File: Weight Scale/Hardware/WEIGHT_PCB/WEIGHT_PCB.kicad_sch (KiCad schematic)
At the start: 0 parts

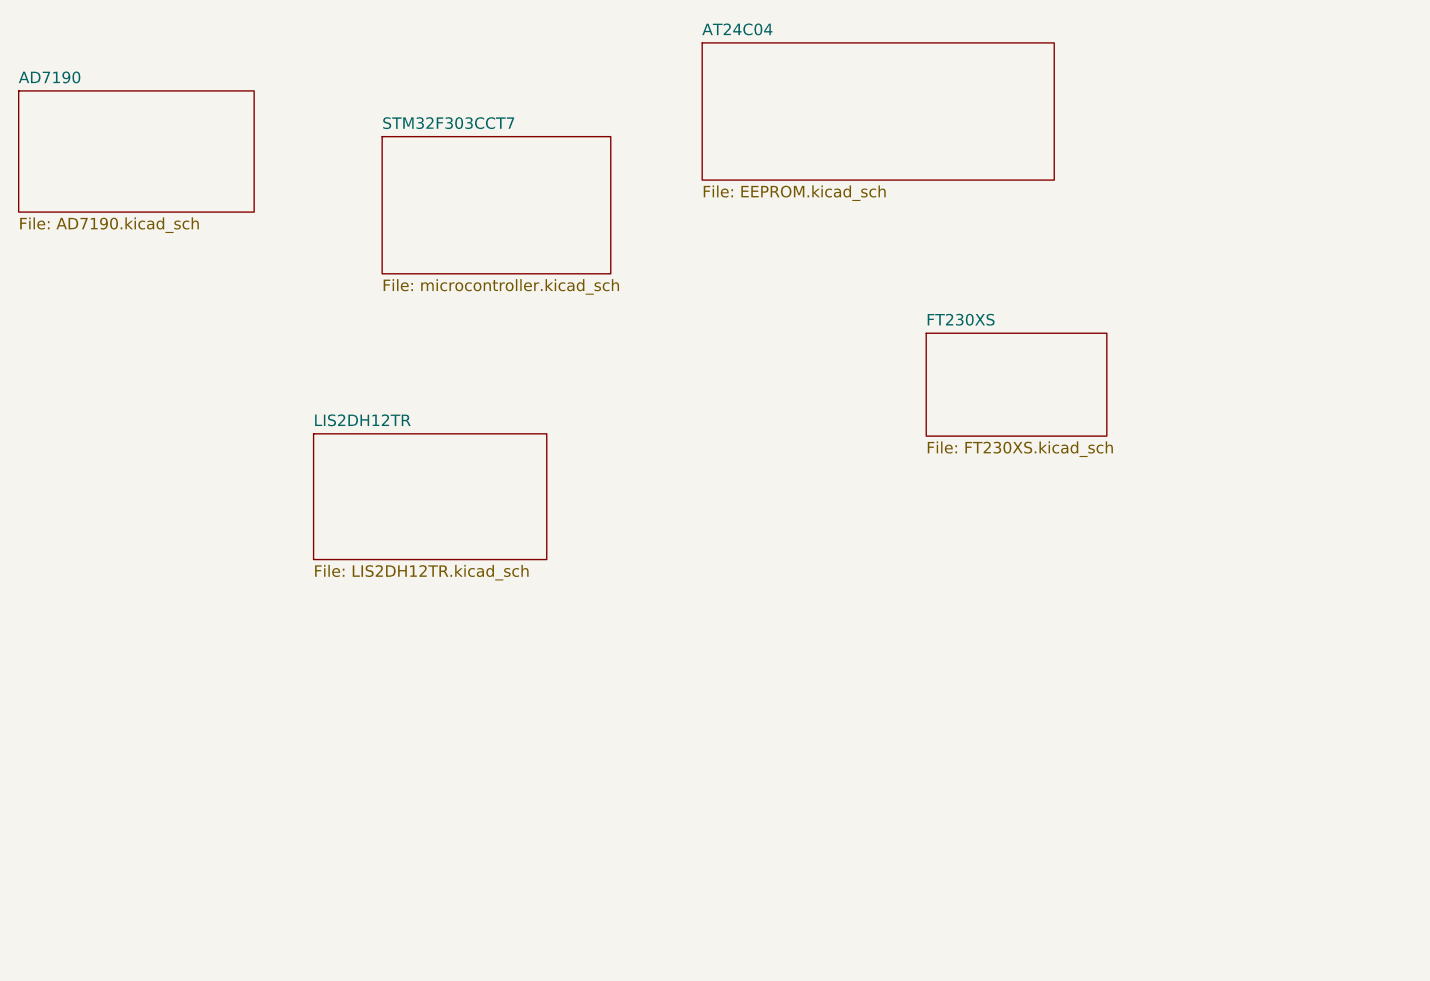
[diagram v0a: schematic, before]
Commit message: update schematics
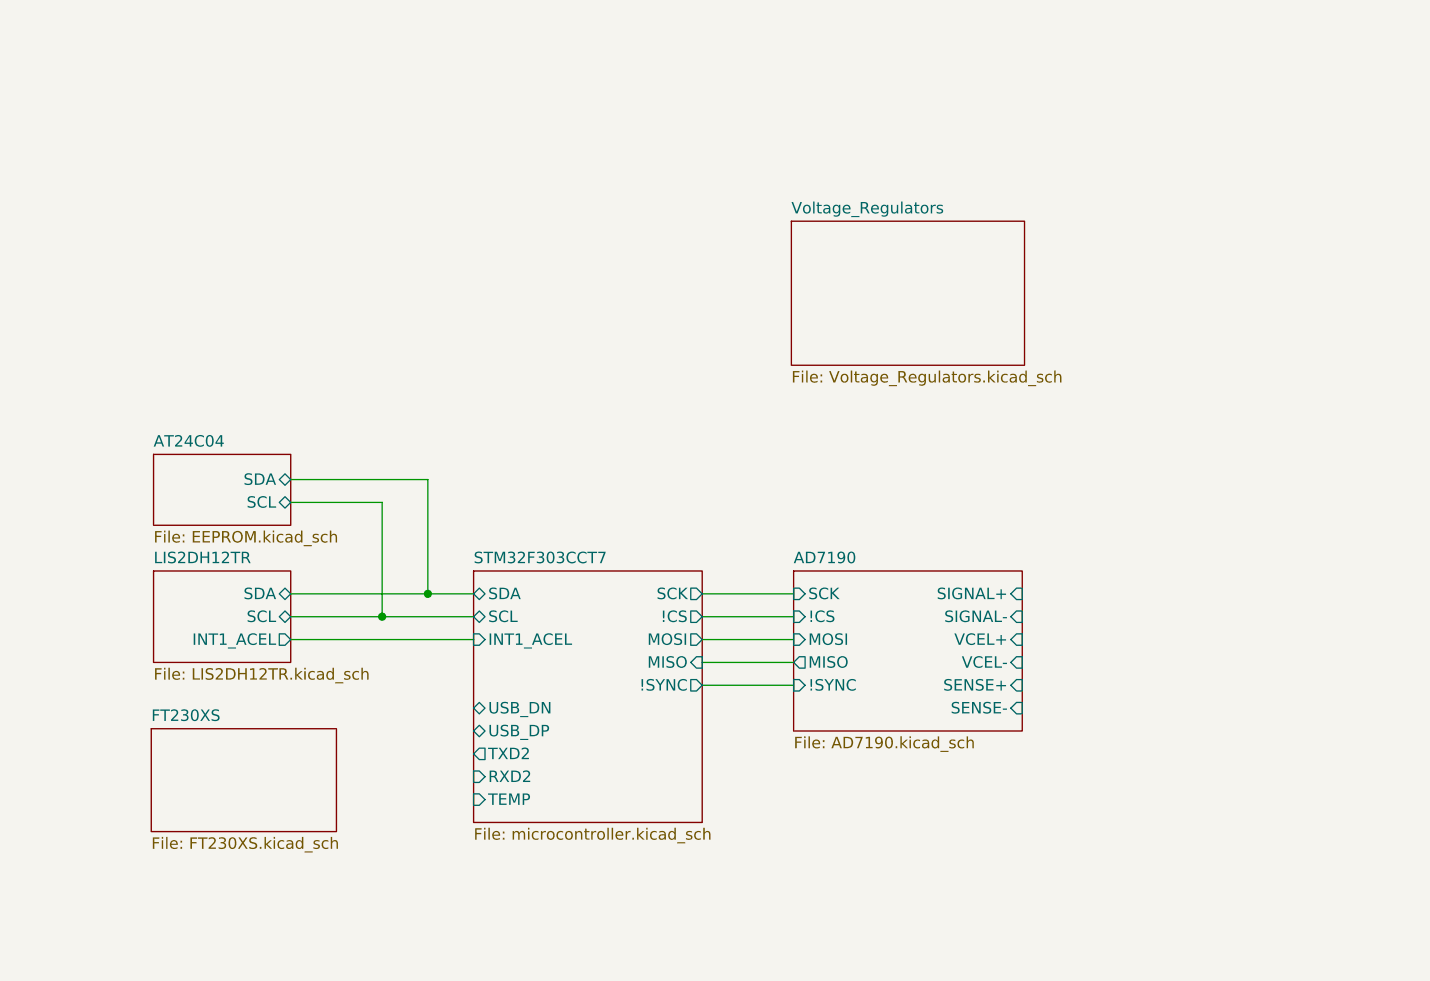
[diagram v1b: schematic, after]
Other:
- added sheet Voltage_Regulators (Voltage_Regulators.kicad_sch)
- sheet AD7190 ports: added !CS, !SYNC, MISO, MOSI, SCK, SENSE+, SENSE-, SIGNAL+, SIGNAL-, VCEL+, VCEL-; removed none
- sheet AT24C04 ports: added SCL, SDA; removed none
- sheet LIS2DH12TR ports: added INT1_ACEL, SCL, SDA; removed none
- sheet STM32F303CCT7 ports: added !CS, !SYNC, INT1_ACEL, MISO, MOSI, RXD2, SCK, SCL, SDA, TEMP, TXD2, USB_DN, USB_DP; removed none

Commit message: update schematics
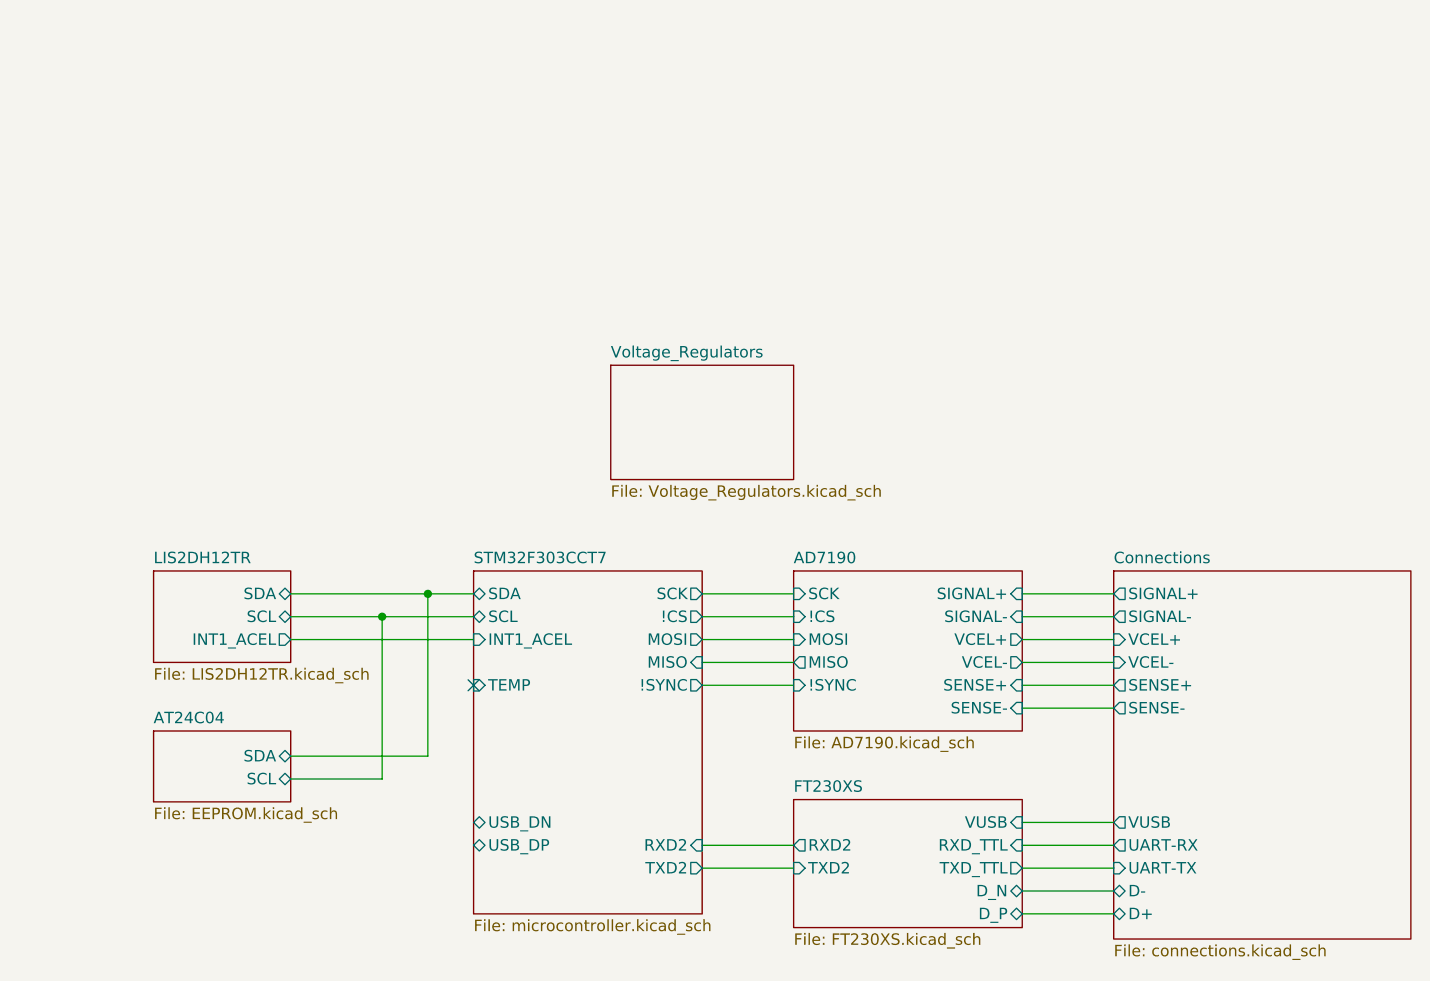
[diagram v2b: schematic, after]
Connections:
- no-connect marks 0 -> 1
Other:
- added sheet Connections (connections.kicad_sch)
- sheet FT230XS ports: added D_N, D_P, RXD2, RXD_TTL, TXD2, TXD_TTL, VUSB; removed none
